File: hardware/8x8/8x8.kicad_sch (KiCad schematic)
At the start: 11 parts

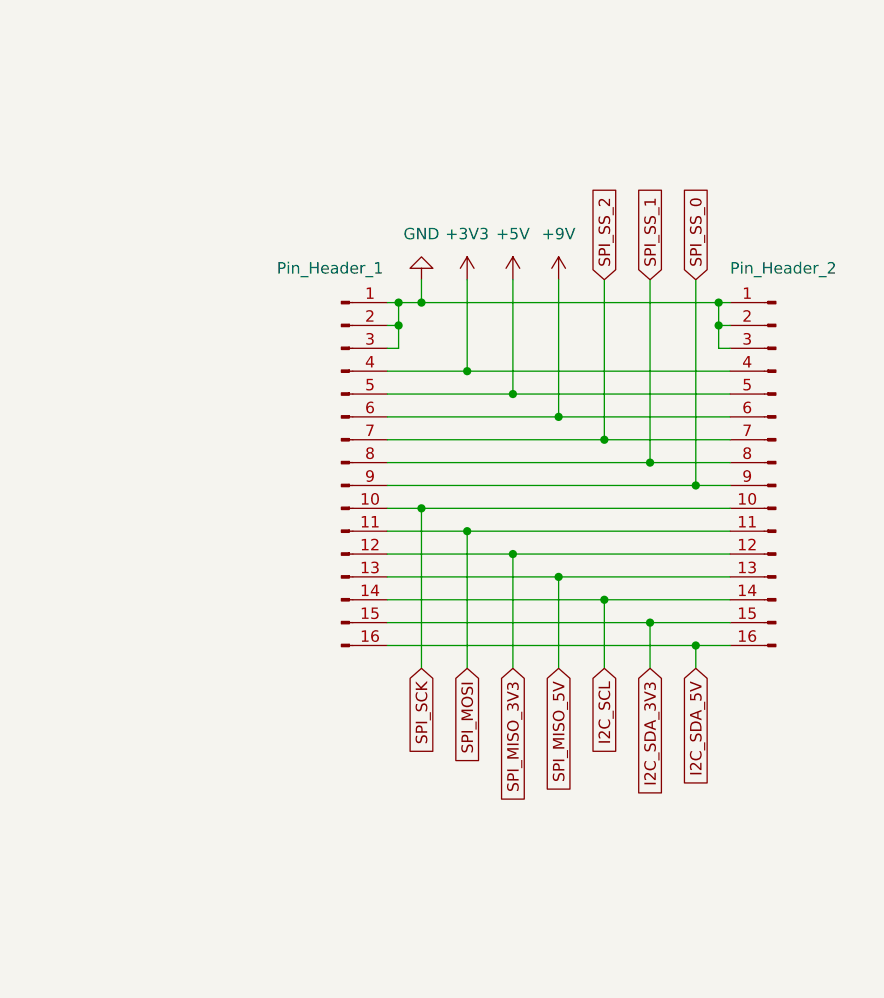
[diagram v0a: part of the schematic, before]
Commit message: Updated Pin Headers
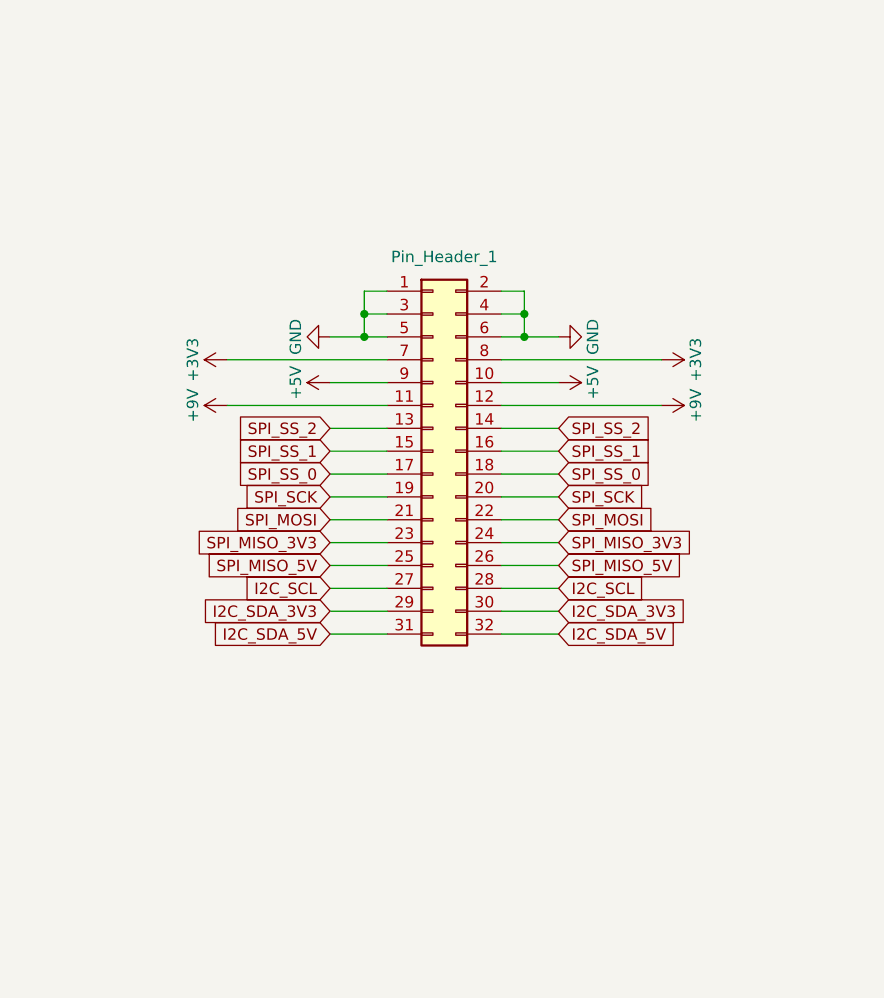
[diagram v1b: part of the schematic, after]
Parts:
- removed Pin_Header_1, Pin_Header_2: Conn_01x16_Male, symbol Connector:Conn_01x16_Male
- added Pin_Header_1: Conn_02x16_Odd_Even, Connector_PinHeader_2.54mm:PinHeader_2x16_P2.54mm_Vertical, symbol Connector_Generic:Conn_02x16_Odd_Even
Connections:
- net +3V3: now also Pin_Header_1.7 (Pin_7), Pin_Header_1.8 (Pin_8)
- net +5V: now also Pin_Header_1.10 (Pin_10), Pin_Header_1.9 (Pin_9)
- net +9V: now also Pin_Header_1.11 (Pin_11), Pin_Header_1.12 (Pin_12)
- net GND: now also Pin_Header_1.1 (Pin_1), Pin_Header_1.2 (Pin_2), Pin_Header_1.3 (Pin_3), Pin_Header_1.4 (Pin_4), Pin_Header_1.5 (Pin_5), Pin_Header_1.6 (Pin_6)
- net I2C_SCL: now also Pin_Header_1.27 (Pin_27), Pin_Header_1.28 (Pin_28)
- net I2C_SDA_3V3: now also Pin_Header_1.29 (Pin_29), Pin_Header_1.30 (Pin_30)
- net I2C_SDA_5V: now also Pin_Header_1.31 (Pin_31), Pin_Header_1.32 (Pin_32)
- net SPI_MISO_3V3: now also Pin_Header_1.23 (Pin_23), Pin_Header_1.24 (Pin_24)
- net SPI_MISO_5V: now also Pin_Header_1.25 (Pin_25), Pin_Header_1.26 (Pin_26)
- net SPI_MOSI: now also Pin_Header_1.21 (Pin_21), Pin_Header_1.22 (Pin_22)
- net SPI_SCK: now also Pin_Header_1.19 (Pin_19), Pin_Header_1.20 (Pin_20)
- net SPI_SS_0: now also Pin_Header_1.17 (Pin_17), Pin_Header_1.18 (Pin_18)
- net SPI_SS_1: now also Pin_Header_1.15 (Pin_15), Pin_Header_1.16 (Pin_16)
- net SPI_SS_2: now also Pin_Header_1.13 (Pin_13), Pin_Header_1.14 (Pin_14)
